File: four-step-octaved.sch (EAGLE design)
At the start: 29 parts, among them IC1 556, IC2 4017N, IC3 4040N, U1 LM386N

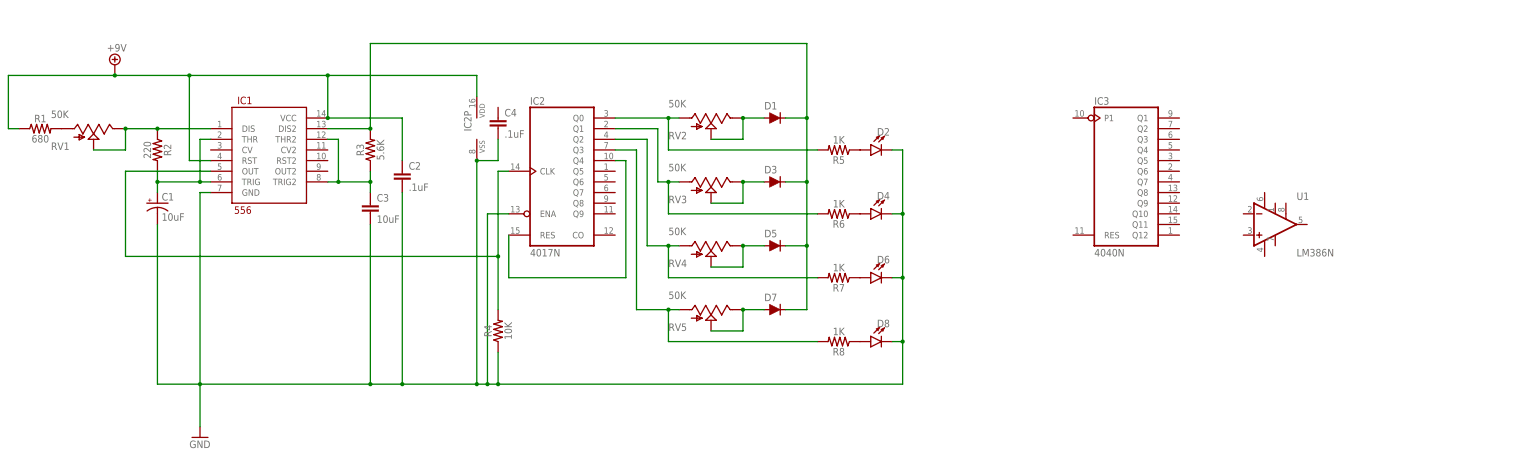
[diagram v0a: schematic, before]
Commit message: Add 4040 and 386
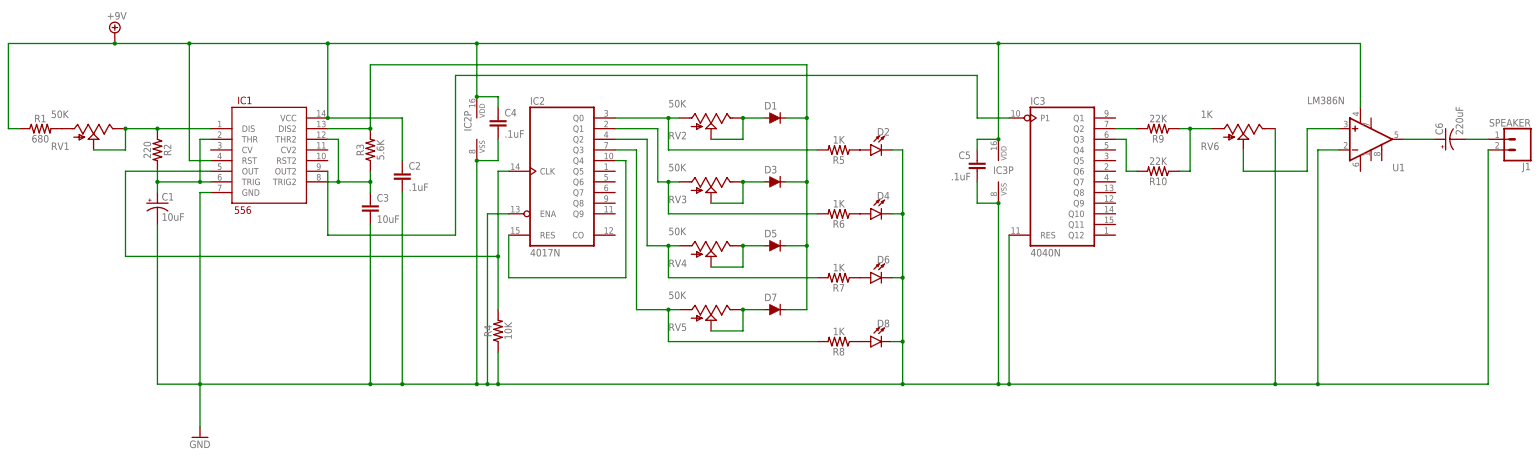
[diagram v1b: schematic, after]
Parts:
- added C5: .1uF, SparkFun-Capacitors:0.1UF-KIT-EZ-50V-20%
- added C6: 220uF, SparkFun-Capacitors:100UF-POLAR-RADIAL-2.5MM-25V-20%
- added J1: SPEAKER, SparkFun-Connectors:CONN_02
- added R10, R9: 22K, SparkFun-Resistors:1KOHM-HORIZ-1/4W-1%
- added RV6: 1K, SparkFun-Retired:POTTRIM
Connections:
- new net N$20: IC3A.Q2, R9.2
- new net N$21: IC1.OUT2, IC3A.P1
- new net N$22: IC3A.Q3, R10.2
- new net N$23: R10.1, R9.1, RV6.A
- new net N$24: RV6.S, U1.+IN
- new net N$27: C6.-, J1.1
- new net N$28: C6.+, U1.OUT
- net +9V: now also C4.1, C5.1, IC3P.VDD, U1.V-
- net GND: now also C5.2, IC3A.RES, IC3P.VSS, J1.2, RV6.E, U1.-IN
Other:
- moved on the sheet: IC3, U1
